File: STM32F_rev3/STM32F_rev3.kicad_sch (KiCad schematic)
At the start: 62 parts, among them J1 USB_B, J2 Tag connect, Q8 SS8050, Q9 SS8050, SW1 SW_Push, U1 MCZ33810EK, U23 PaP_Driver_v1, U24 ADUM4160, U3 STM32F407VGTx, U7 25LCxxx, Y1 25MHz

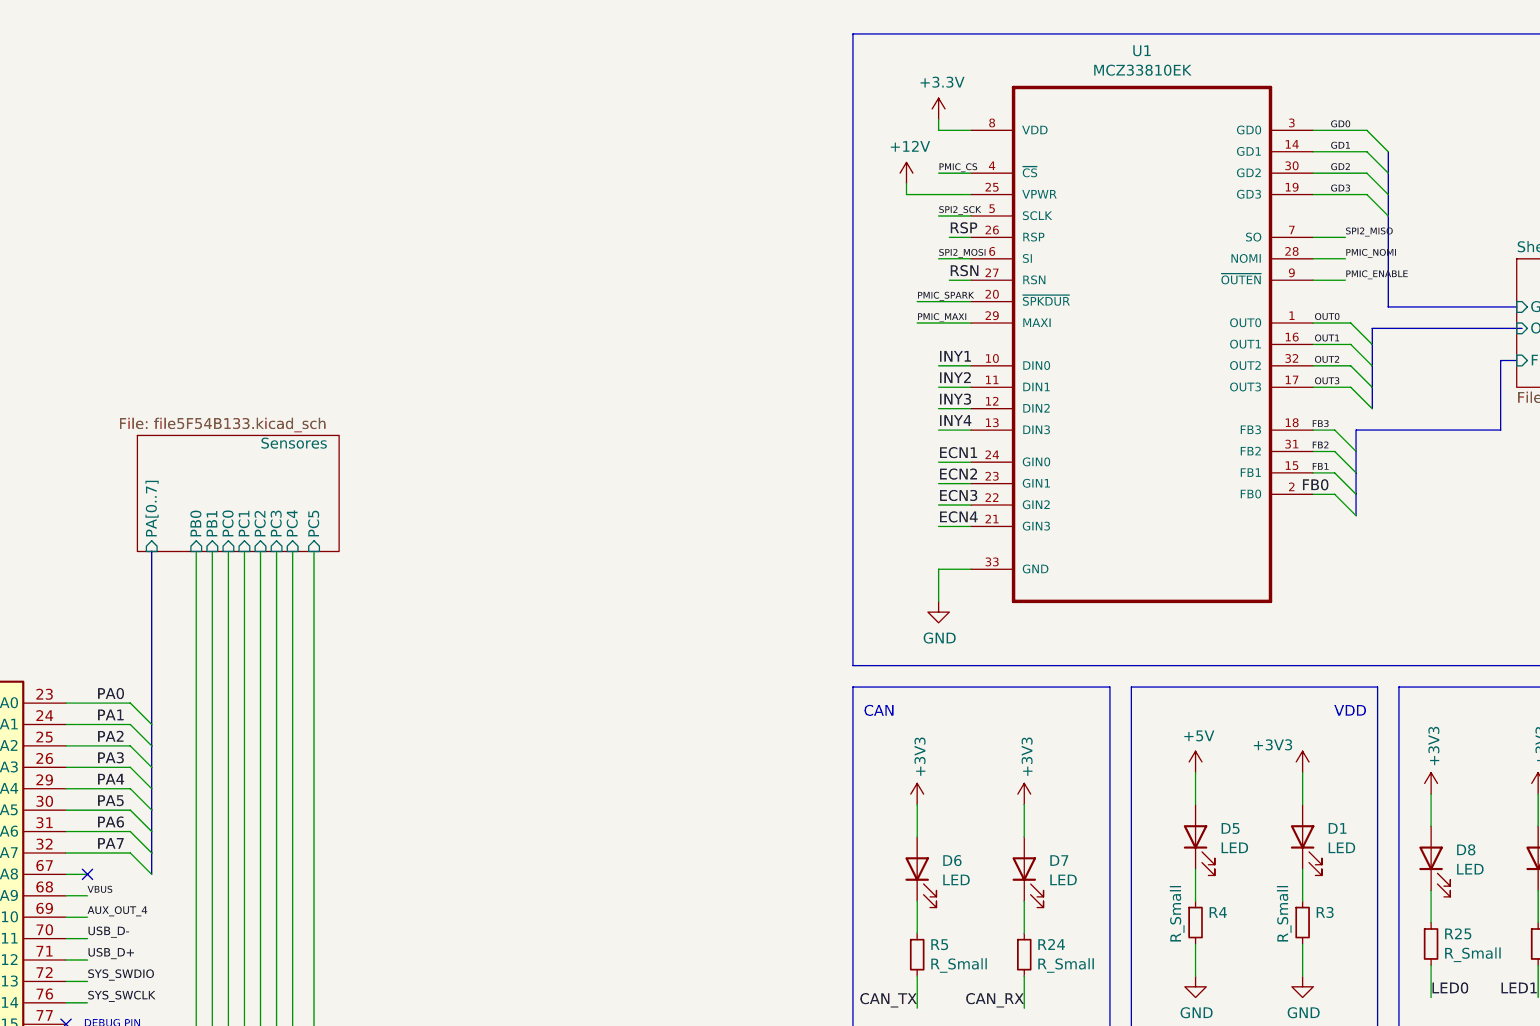
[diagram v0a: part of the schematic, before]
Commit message: Last commit to rev3
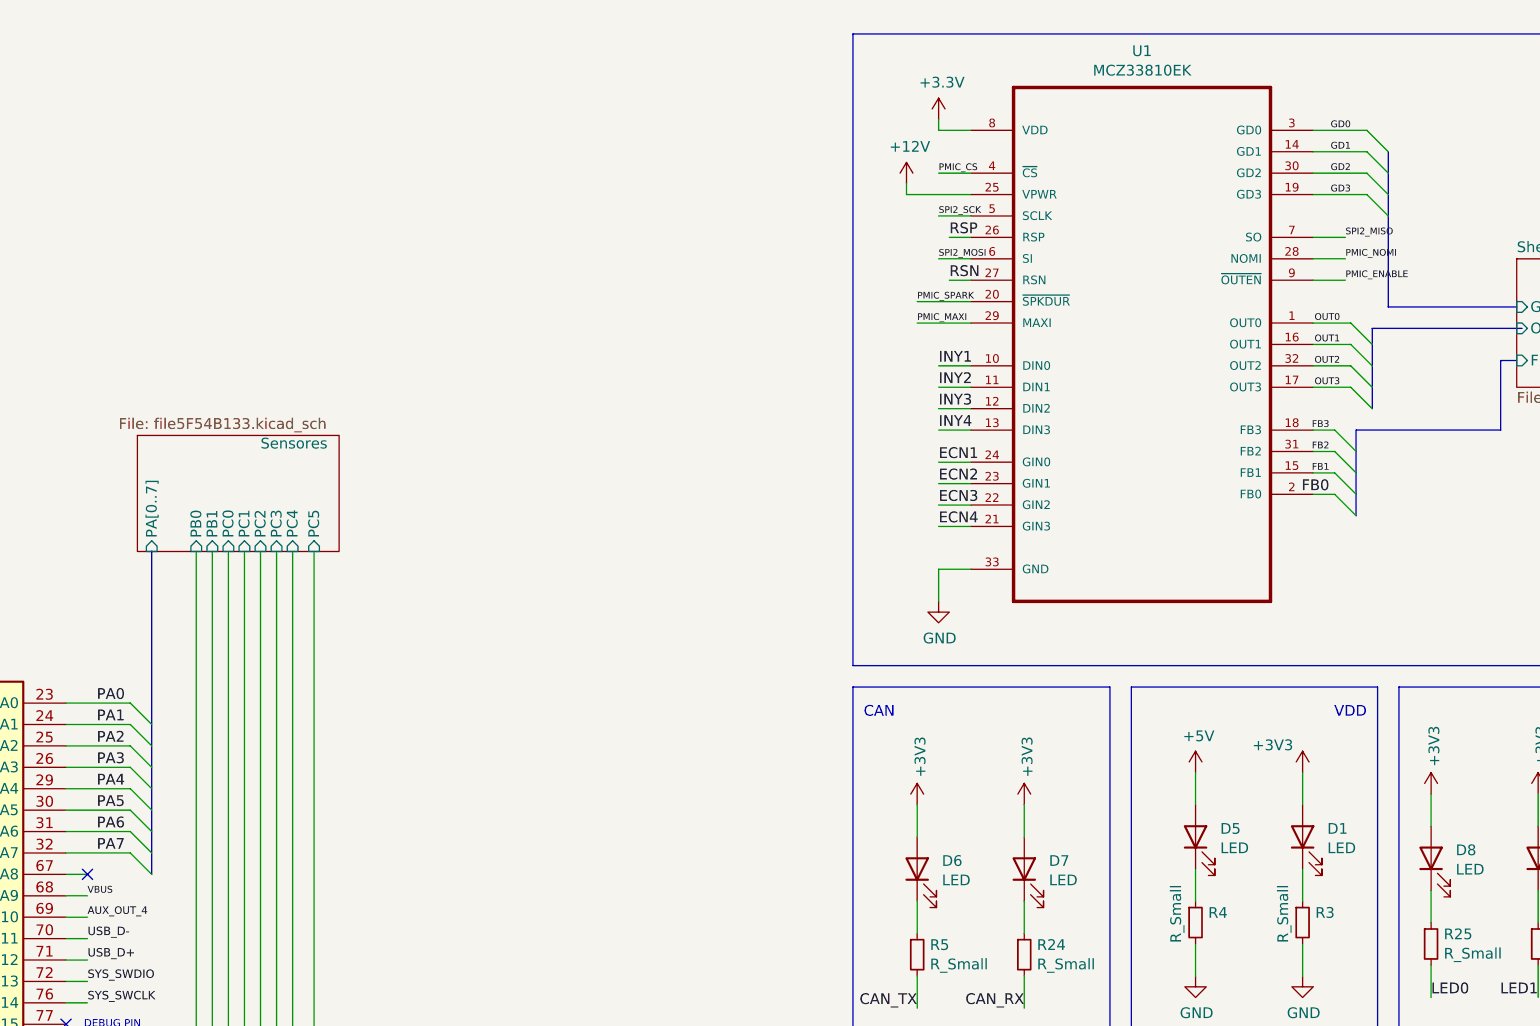
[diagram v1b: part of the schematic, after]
